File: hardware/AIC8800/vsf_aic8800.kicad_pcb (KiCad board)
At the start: 2 copper layers, 27.9 x 50.9 mm, 31 parts, among them J0 USB_C_Receptacle_USB2.0, J1 Conn_01x20, J2 Conn_01x20, J3 Conn_02x05_Counter_Clockwise, Q0 AO3401, Q1 AO3402, SW0 SW_Push, SW1 SW_Push, U0 Module_AIC8800M

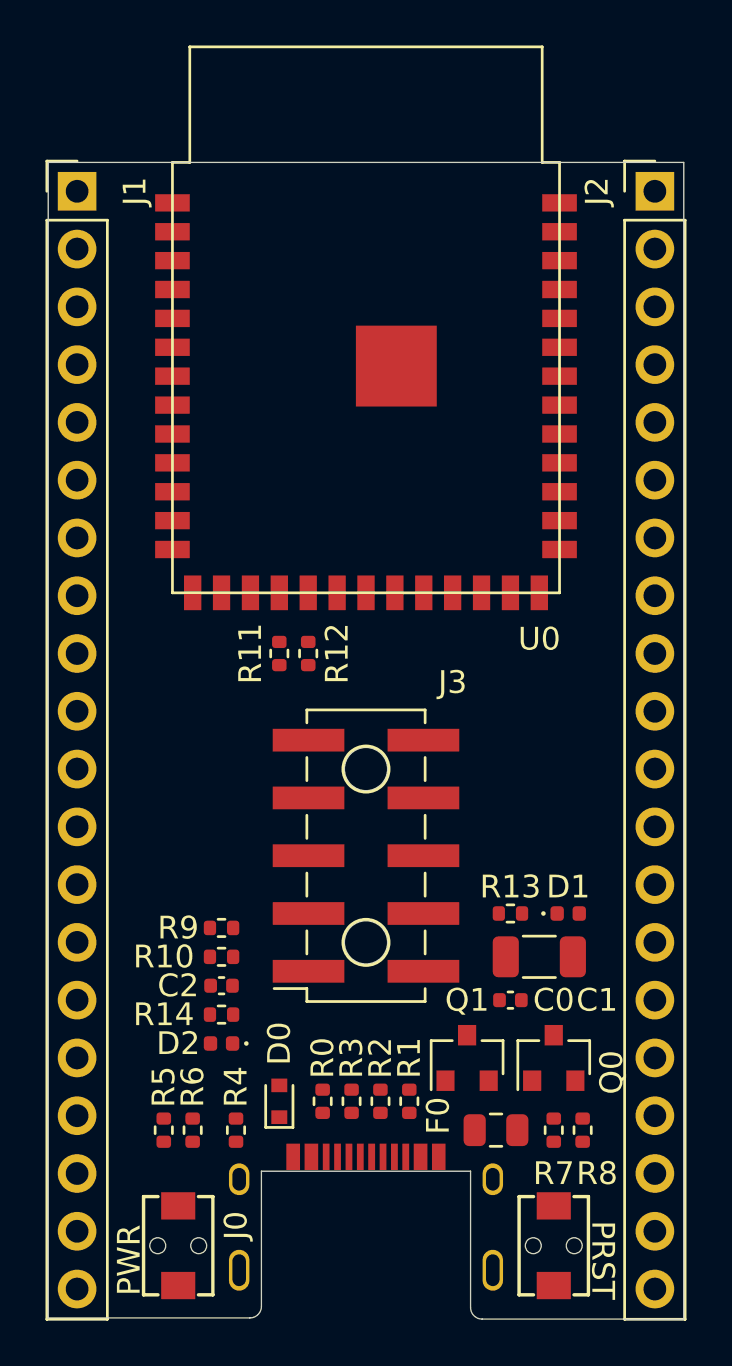
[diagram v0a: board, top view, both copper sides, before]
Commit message: [hardware/aic8800] route
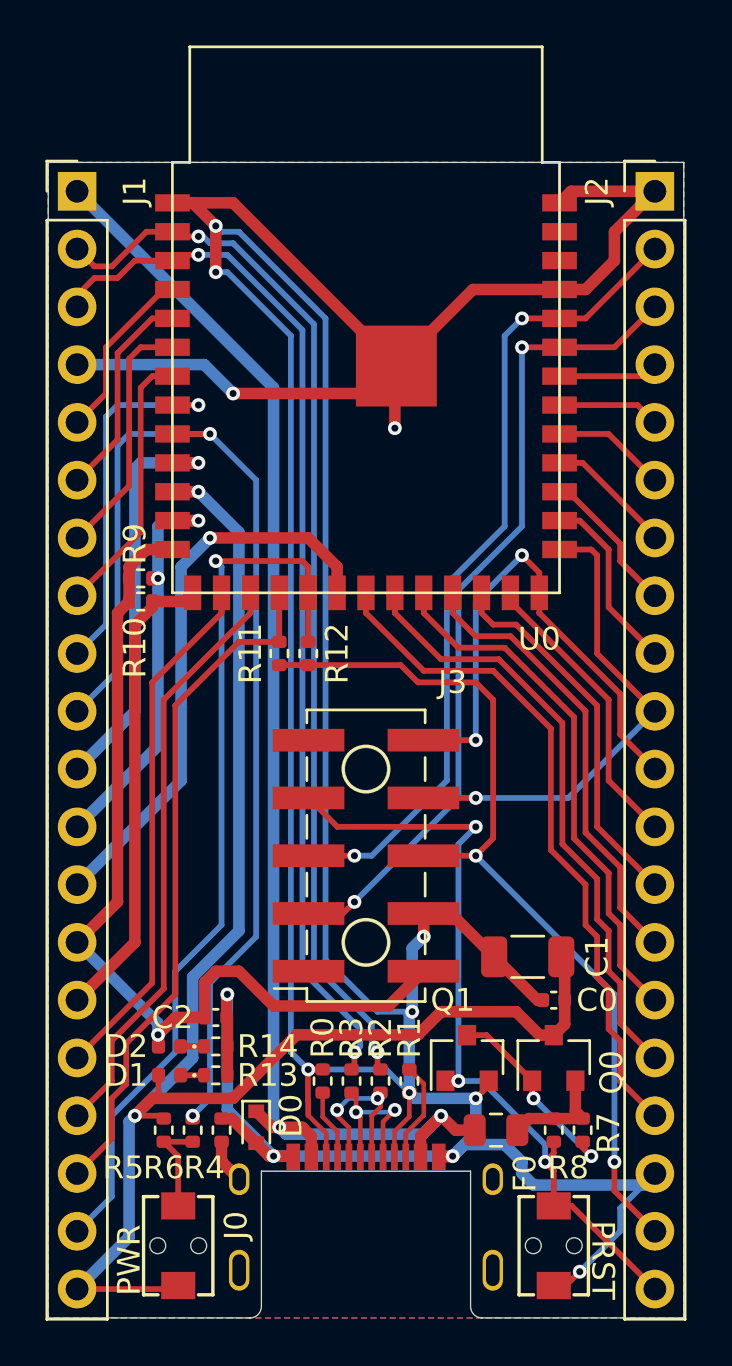
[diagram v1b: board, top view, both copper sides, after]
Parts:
- R13, R14: value 4.7 -> 4.7K
- moved D1 18.9 mm to (208.5, 141.7), turned to 180 degrees
- moved R10 16.0 mm to (207.3, 120.9), turned to 180 degrees
- moved R9 15.8 mm to (207.3, 119.9), turned to 180 degrees
- moved R13 14.8 mm to (210.6, 141.7), turned to 180 degrees
- moved D2 2.29 mm to (208.5, 140.5)
- moved C0 1.91 mm to (225.4, 138.4)
- moved D0 1.53 mm to (212.3, 144.0), turned to 270 degrees
- moved C2 1.42 mm to (210.6, 139.2)
- moved R14 1.42 mm to (210.6, 140.5), turned to 180 degrees
- moved R7 1.27 mm to (226.7, 144.1), turned to 270 degrees
- moved R8 1.27 mm to (225.4, 144.1)
- moved R0 0.89 mm to (215.3, 142.0)
- moved R1 0.89 mm to (219.1, 142.0), turned to 90 degrees
- moved R2 0.89 mm to (217.8, 142.0)
- moved R3 0.89 mm to (216.5, 142.0)
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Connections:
- J1 pad 12: /VSYS -> /V18
- J1 pad 13: /V18 -> /V09
- J1 pad 20: /V09 -> /VSYS
- J2 pad 19: /PRST -> /DL
- J2 pad 20: /DL -> /PRST
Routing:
- net GND: track 0.00 -> 207.4 mm, vias 0 -> 13
- net /VSYS: track 0.00 -> 72.4 mm, vias 0 -> 2
- net /USB_5V: track 0.00 -> 60.1 mm, vias 0 -> 2
- net /PKEY: track 0.00 -> 50.4 mm, vias 0 -> 2
- net /USB_DM: track 0.00 -> 47.0 mm, vias 0 -> 2
- net /USB_DP: track 0.00 -> 46.2 mm, vias 0 -> 2
- net /VCC: track 0.00 -> 40.7 mm, vias 0 -> 1
- net /B7: track 0.00 -> 39.7 mm, vias 0 -> 1
- net /DL: track 0.00 -> 39.3 mm, vias 0 -> 2
- net /A0: track 0.00 -> 36.2 mm, vias 0 -> 2
- net /A1: track 0.00 -> 36.2 mm, vias 0 -> 2
- net /PRST: track 0.00 -> 34.8 mm, vias 0 -> 3
- net /B6: track 0.00 -> 30.2 mm
- net /A15: track 0.00 -> 30.0 mm
- net /A14: track 0.00 -> 26.7 mm
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- added copper zone on B.Cu, net GND
- added copper zone on F.Cu, net GND
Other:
- board size 27.9 x 50.9 mm -> 27.9 x 50.8 mm
